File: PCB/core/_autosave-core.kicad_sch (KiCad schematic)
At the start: 10 parts, among them U1 MCU_Seeed_XIAO_ESP32-C3, U2 STP55NF06L

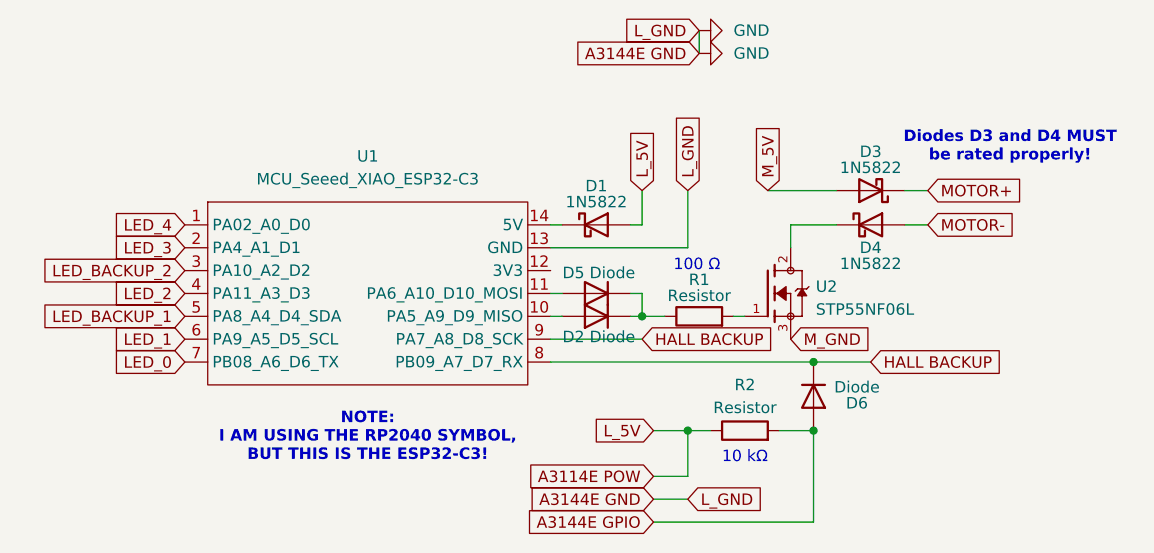
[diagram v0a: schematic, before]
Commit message: licenses!
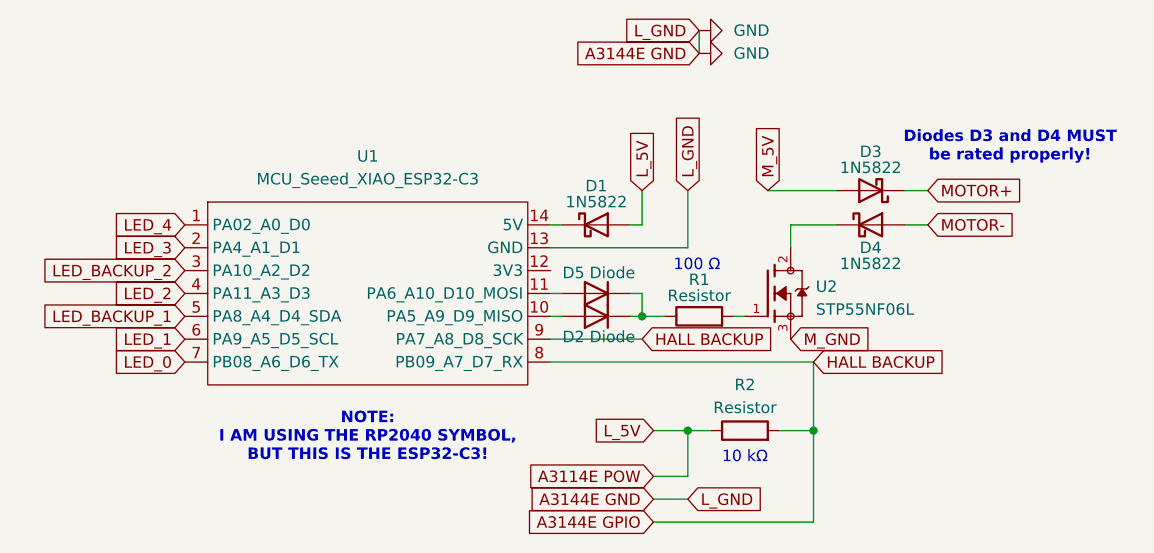
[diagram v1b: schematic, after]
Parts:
- removed D6: Diode, ScottoKeebs_Components:Diode_DO-35, symbol ScottoKeebs:Placeholder_Diode
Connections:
- net HALL BACKUP is gone; now on net A3144E GPIO: U1.8 (PB09_A7_D7_RX), U1.9 (PA7_A8_D8_SCK)
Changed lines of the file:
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@@
 	(paper "A4")
+	(junction
+		(at 104.14 69.85)
+		(diameter 0)
+		(color 0 0 0 0)
+	)
+	(junction
+		(at 99.06 57.15)
+		(diameter 0)
+		(color 0 0 0 0)
+	)
 	(junction
 		(at 118.11 69.85)
@@
 		(color 0 0 0 0)
 	)
-	(junction
-		(at 104.14 69.85)
-		(diameter 0)
-		(color 0 0 0 0)
-	)
-	(junction
-		(at 99.06 57.15)
-		(diameter 0)
-		(color 0 0 0 0)
-	)
-	(junction
-		(at 118.11 62.23)
-		(diameter 0)
-		(color 0 0 0 0)
-	)
 	(wire
 		(pts
@@
 	(wire
 		(pts
+			(xy 118.11 62.23) (xy 118.11 69.85)
+		)
+		(stroke
+			(width 0)
+			(type default)
+		)
+	)
+	(wire
+		(pts
 			(xy 99.06 54.61) (xy 99.06 57.15)
 		)
@@
 		(pts
 			(xy 104.14 69.85) (xy 104.14 74.93)
-		)
-		(stroke
-			(width 0)
-			(type default)
-		)
-	)
-	(wire
-		(pts
-			(xy 124.46 62.23) (xy 118.11 62.23)
 		)
 		(stroke
@@
 	(global_label "HALL BACKUP"
 		(shape input)
-		(at 124.46 62.23 0)
+		(at 118.11 62.23 0)
 		(fields_autoplaced yes)
 		(effects
@@
 		)
 		(property "Intersheetrefs" "${INTERSHEET_REFS}"
-			(at 140.3872 62.23 0)
+			(at 134.0372 62.23 0)
 			(effects
 				(font
@@
 					(unit 1)
 				)
-			)
-		)
-	)
-	(symbol
-		(lib_id "ScottoKeebs:Placeholder_Diode")
-		(at 118.11 66.04 270)
-		(unit 1)
-		(exclude_from_sim no)
-		(in_bom yes)
-		(on_board yes)
-		(dnp no)
-		(property "Reference" "D6"
-			(at 122.936 66.802 90)
-			(effects
-				(font
-					(size 1.27 1.27)
-				)
-			)
-		)
-		(property "Value" "Diode"
-			(at 122.936 65.024 90)
-			(effects
-				(font
-					(size 1.27 1.27)
-				)
-			)
-		)
-		(property "Footprint" "ScottoKeebs_Components:Diode_DO-35"
-			(at 118.11 66.04 0)
-			(effects
-				(font
-					(size 1.27 1.27)
-				)
-				(hide yes)
-			)
-		)
-		(property "Datasheet" ""
-			(at 118.11 66.04 0)
-			(effects
-				(font
-					(size 1.27 1.27)
-				)
-				(hide yes)
-			)
-		)
-		(property "Description" "1N4148 (DO-35) or 1N4148W (SOD-123)"
-			(at 118.11 66.04 0)
-			(effects
-				(font
-					(size 1.27 1.27)
-				)
-				(hide yes)
-			)
-		)
-		(property "Sim.Device" "D"
-			(at 118.11 66.04 0)
-			(effects
-				(font
-					(size 1.27 1.27)
-				)
-				(hide yes)
-			)
-		)
-		(property "Sim.Pins" "1=K 2=A"
-			(at 118.11 66.04 0)
-			(effects
-				(font
-					(size 1.27 1.27)
-				)
-				(hide yes)
-			)
-		)
-		(pin "1"
-		)
-		(pin "2"
-		)
-		(instances
-			(project "core"
-				(path "/fbd72b7d-ff34-44b4-b2bb-0e63eec67b9d"
-					(reference "D6")
-					(unit 1)
-				)
